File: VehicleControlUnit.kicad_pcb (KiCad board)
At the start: 2 copper layers, 86.6 x 100 mm, 101 parts, among them Con1 LED, Con2 LED, J1 Conn_01x02, J10 Conn_01x04, J11 Conn_01x04, J14 SFH11-PBPC-D05-ST-BK, J15 SFH11-PBPC-D05-ST-BK, J2 Conn_01x02, J3 Conn_01x02, J5 SFH11-PBPC-D05-ST-BK, J6 SFH11-PBPC-D05-ST-BK, J7 Conn_01x04, J8 Conn_01x04, J9 USB_C_Receptacle_USB2.0_16P, Q1 PSMN8R5-40MSDX, Q2 IRLML0030, Q3 IRLML0030, SW1 RESET, SW2 BOOT, U1 LM74501-Q1, U2 TLV1117LV33DCYR, U4 ESP32-C6-MINI-1/U, U5 TCMT1106, U6 TCMT1106

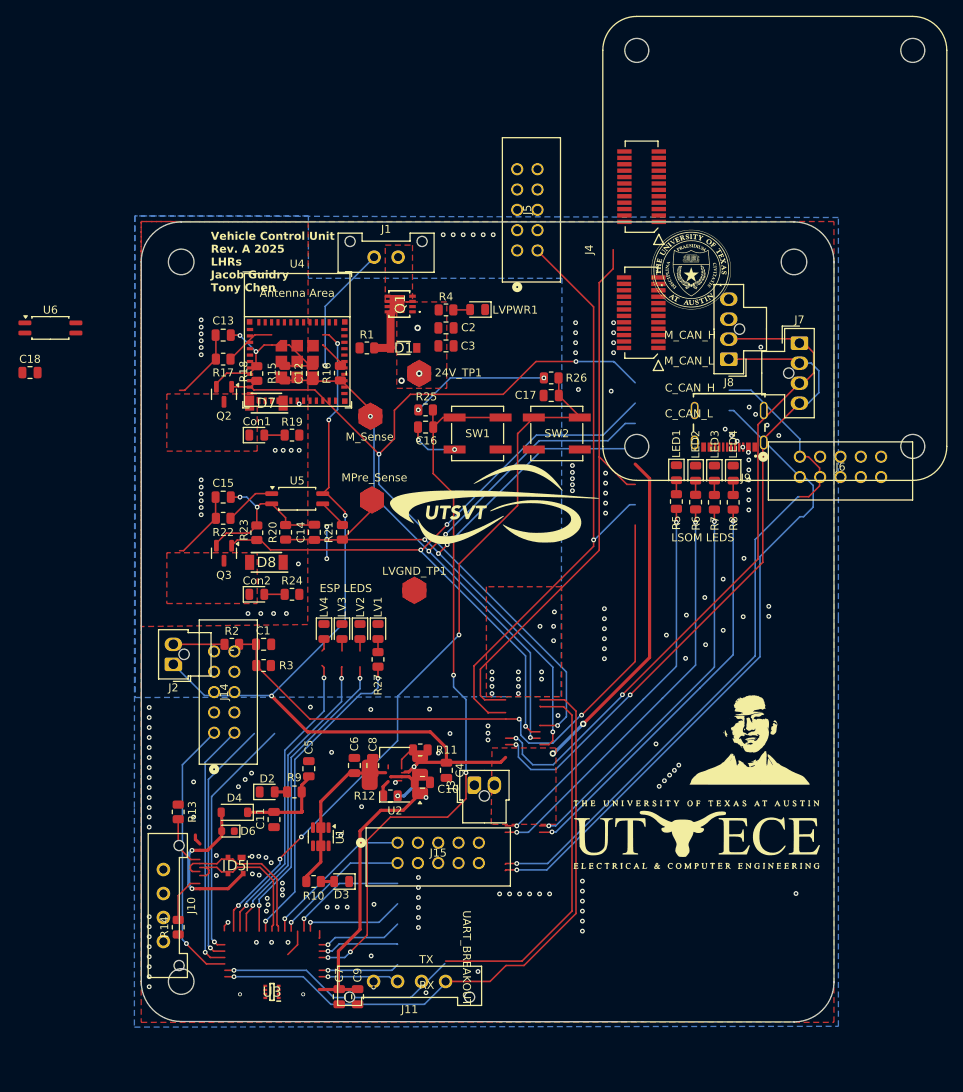
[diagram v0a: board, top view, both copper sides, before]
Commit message: routing done
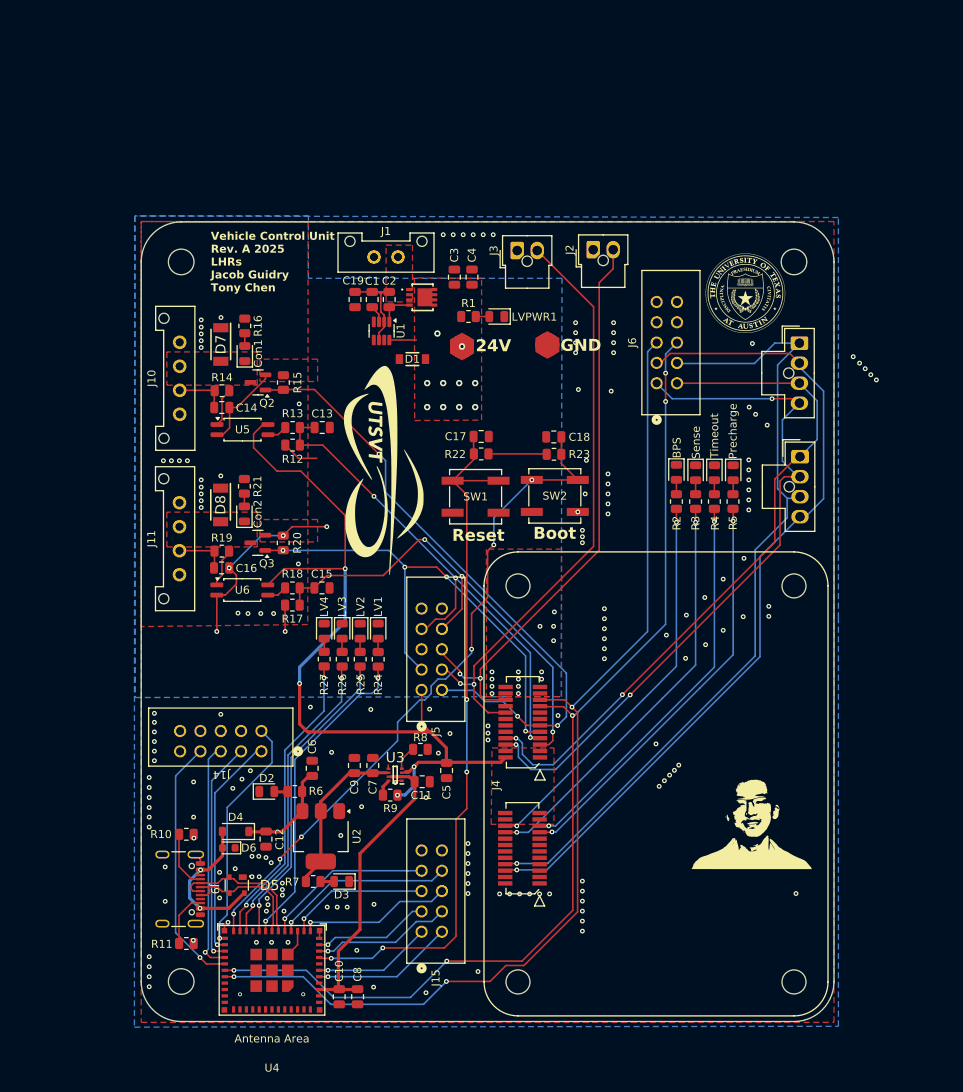
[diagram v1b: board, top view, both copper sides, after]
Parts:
- removed M_Pre_Sen_TP1, M_Sen_TP1: TestPoint, UTSVT_Special:TestPoint_HEX_3mmID
- added C19: 0.1u, Capacitor_SMD:C_0805_2012Metric, F.Cu at (136.0, 51.5)
- added G***: LHRs_LOGO, UTSVT_Logos:LHRs_LOGO, F.Cu at (120.0, 96.8)
- G***: moved to B.Cu
- J2, J3: footprint Connector_Molex:Molex_Nano-Fit_105309-xx02_1x02_P2.50mm_Vertical -> UTSVT_Connectors:Molex_Nano-Fit_105309-xx02_1x02_P2.50mm_Vertical
- J7, J8: footprint Connector_Molex:Molex_Nano-Fit_105309-xx04_1x04_P2.50mm_Vertical -> UTSVT_Connectors:Molex_Nano-Fit_105309-xx04_1x04_P2.50mm_Vertical
- J9: footprint UTSVT_Connectors:GCT_USB4215-03-A_REVA -> UTSVT_Connectors:USB_C_Receptacle_GCT_USB4105-xx-A_16P_TopMnt_Horizontal
- moved J9 91.9 mm to (113.0, 125.2), turned to -90 degrees
- moved U4 81.6 mm to (125.6, 138.1), turned to 180 degrees
- moved G*** 74.1 mm to (140.0, 55.0), turned to 180 degrees
- moved J2 73.8 mm to (165.8, 45.3), turned to 90 degrees
- moved R7 69.0 mm to (130.8, 124.3), turned to 0 degrees
- moved J4 68.6 mm to (150.9, 112.3)
- moved R14 67.3 mm to (119.3, 63.0), turned to 0 degrees
- moved J3 67.0 mm to (156.2, 45.4)
- moved C18 66.0 mm to (160.8, 68.7), turned to 180 degrees
- moved U1 63.7 mm to (139.3, 55.5)
- moved R6 61.8 mm to (128.4, 113.0), turned to 180 degrees
- moved C4 61.7 mm to (150.6, 48.8), turned to 90 degrees
- moved J11 60.8 mm to (114.0, 86.0), turned to 90 degrees
- moved C12 58.5 mm to (124.8, 119.0)
- moved R2 58.4 mm to (176.2, 76.8), turned to 90 degrees
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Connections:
- J14 pad 1: /ESP/IO1 -> /ESP/IO4
- J14 pad 2: /ESP/IO2 -> /ESP/IO13
- J14 pad 4: /ESP/IO4 -> unconnected-(J14-Pad4)
- J14 pad 5: /ESP/IO5 -> /ESP/IO2
- J14 pad 6: /ESP/IO6 -> unconnected-(J14-Pad6)
- J14 pad 7: /ESP/IO7 -> /ESP/IO1
- J14 pad 8: /ESP/IO8 -> unconnected-(J14-Pad8)
- J14 pad 9: /ESP/IO9 -> GND
- J15 pad 1: /ESP/IO10 -> /ESP/IO11
- J15 pad 2: /ESP/IO11 -> /ESP/IO12
- J15 pad 3: /ESP/IO12 -> /ESP/IO9
- J15 pad 4: /ESP/IO13 -> /ESP/IO10
- J15 pad 5: /ESP/USB_D+ -> /ESP/IO7
- J15 pad 6: /ESP/USB_D- -> /ESP/IO8
- J15 pad 7: unconnected-(J15-Pad7) -> /ESP/IO5
- J15 pad 8: unconnected-(J15-Pad8) -> /ESP/IO6
- J15 pad 9: unconnected-(J15-Pad9) -> GND
- J5 pad 1: /M_Enable -> 3V3_LSOM
- J5 pad 2: /MPre_Enable -> /M_Enable
- J5 pad 3: /M_Sense -> /MPre_Enable
- J5 pad 4: /MPre_Sense -> /VPrecharge-
- J5 pad 7: /VPrecharge- -> /M_Sense
- J5 pad 8: /Precharge_Ready -> /MPre_Sense
- J5 pad 9: unconnected-(J5-Pad9) -> GND
- J6 pad 5: /ESP_RX -> /ESP_TX
- J6 pad 6: /ESP_TX -> /ESP_RX
- J6 pad 9: unconnected-(J6-Pad9) -> GND
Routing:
- net /ESP_TX: track 0.00 -> 130.6 mm, vias 0 -> 3
- net /MPre_Enable: track 165.3 -> 63.0 mm
- net +24V: track 87.4 -> 3.36 mm, vias 40 -> 46
- net /ESP_RX: track 47.4 -> 131.0 mm, vias 0 -> 5
- net /Precharge_Ready: track 78.5 -> 0.00 mm, vias 2 -> 0
- net /VPrecharge-: track 0.00 -> 74.6 mm, vias 0 -> 2
- net /LED2: track 0.00 -> 51.9 mm, vias 0 -> 2
- net /ESP/5V_USB: track 64.0 -> 12.6 mm, vias 2 -> 0
- net /LED3: track 0.00 -> 49.8 mm, vias 0 -> 2
- net /ESP/3V3_USB: track 70.1 -> 20.4 mm, vias 2 -> 0
- net /LED1: track 0.00 -> 49.4 mm, vias 0 -> 2
- net Net-(U3-!ON): track 51.6 -> 3.07 mm, vias 2 -> 0
- net 3V3_LSOM: track 153.8 -> 105.7 mm, vias 8 -> 4
- net /ESP/LED1: track 0.00 -> 40.1 mm, vias 0 -> 2
- net /ESP/LED4: track 77.7 -> 37.7 mm, vias 4 -> 2
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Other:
- outline, holes or cut-outs redrawn
- board text added: "24V"
- board text added: "BPS"
- board text added: "Boot"
- board text added: "GND"
- board text added: "Precharge"
- board text added: "Reset"
- board text added: "Sense"
- board text added: "Timeout"
- board text removed: "C_CAN_H C_CAN_L"
- board text removed: "ESP LEDS"
- board text removed: "LSOM LEDS"
- board text removed: "MPre_Sense"
- board text removed: "M_CAN_H M_CAN_L"
- board text removed: "M_Sense"
- board text removed: "TX RX"
- board text removed: "UART_BREAKOUT"
